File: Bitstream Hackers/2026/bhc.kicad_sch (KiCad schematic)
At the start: 7 parts, among them U1 AT24CS01-SSHM

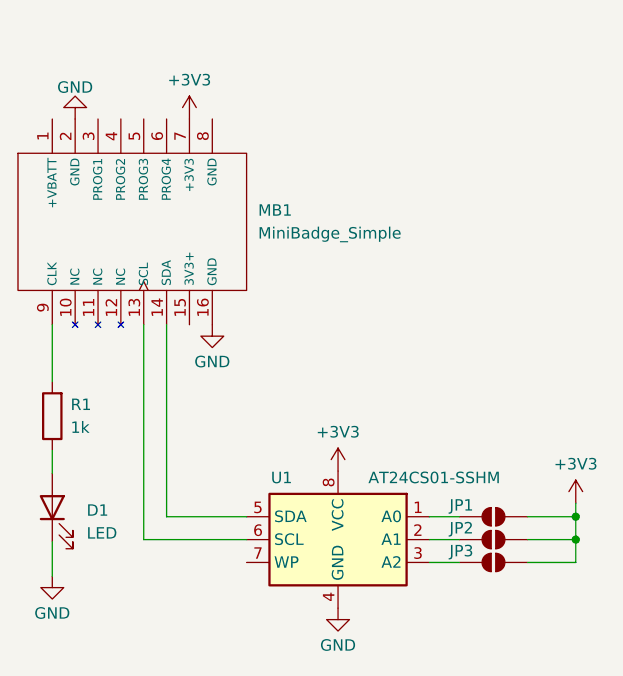
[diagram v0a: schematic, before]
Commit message: Adding finals, gerbers
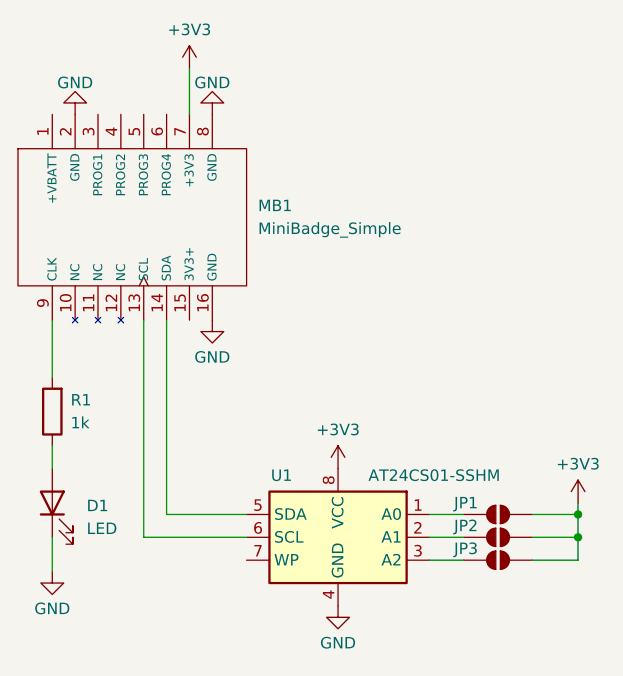
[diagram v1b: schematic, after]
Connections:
- net GND: now also MB1.8 (GND)
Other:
- moved on the sheet: D1, JP1, JP2, JP3, MB1, R1
